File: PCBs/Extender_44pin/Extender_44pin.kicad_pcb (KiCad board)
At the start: 2 copper layers, 119.1 x 224.9 mm, 46 parts, among them J10 J, J11 K, J12 L, J13 M, J14 N, J15 P, J16 R, J17 S, J18 T, J19 U, J20 V, J21 W, J22 X, J23 1, J24 2, J25 3, J26 4, J27 5, J28 6, J29 7, J3 A, J30 8, J31 9, J32 10, J33 11, J34 12, J35 13, J36 14, J37 15, J38 16, J39 17, J4 B, J40 18, J41 19, J42 20, J43 21, J44 22, J45 Y, J46 Z, J5 C, J6 D, J7 E, J8 F, J9 H

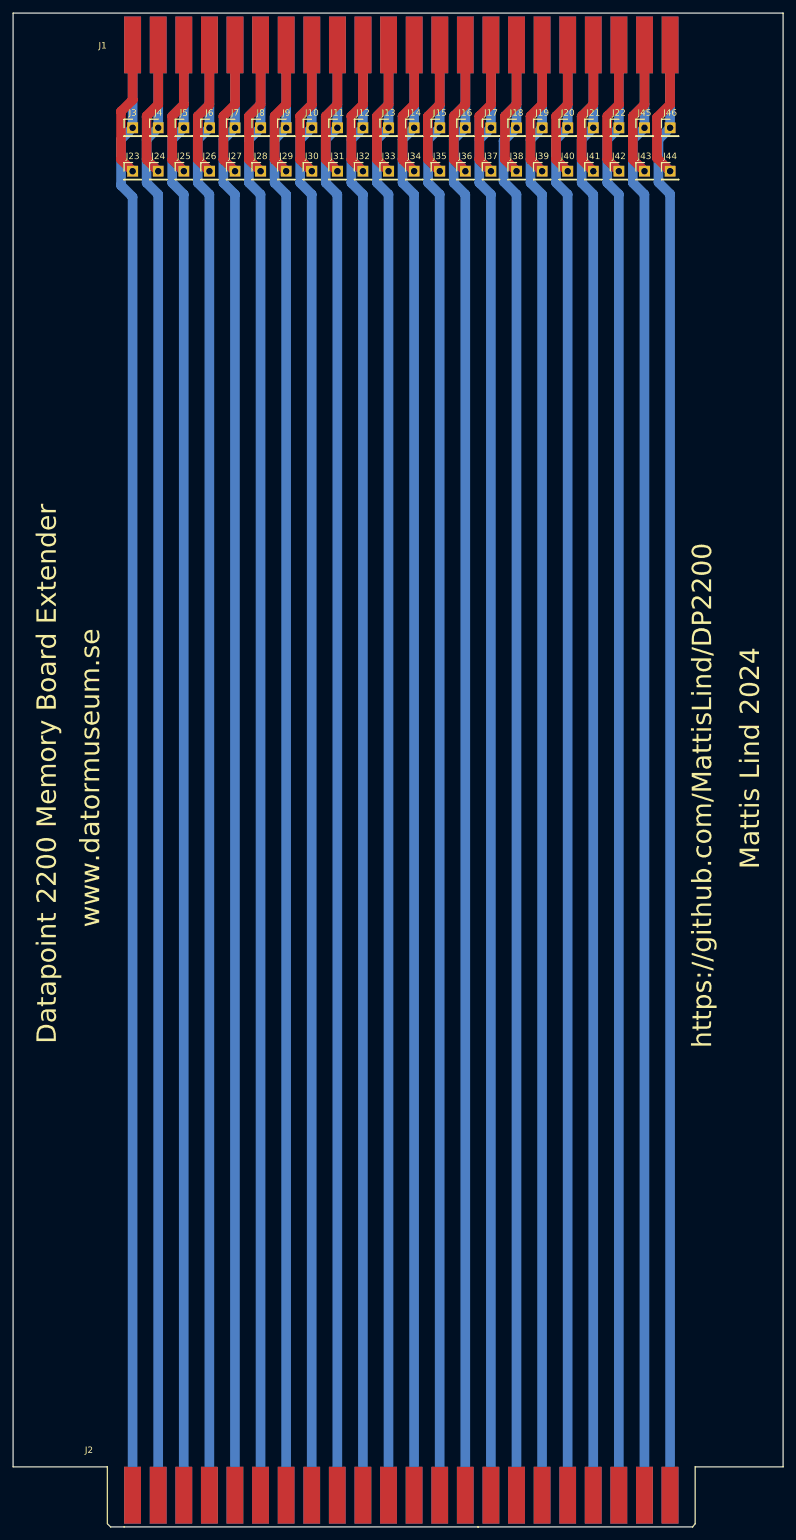
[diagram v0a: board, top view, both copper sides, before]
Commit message: Updates of extender boards.
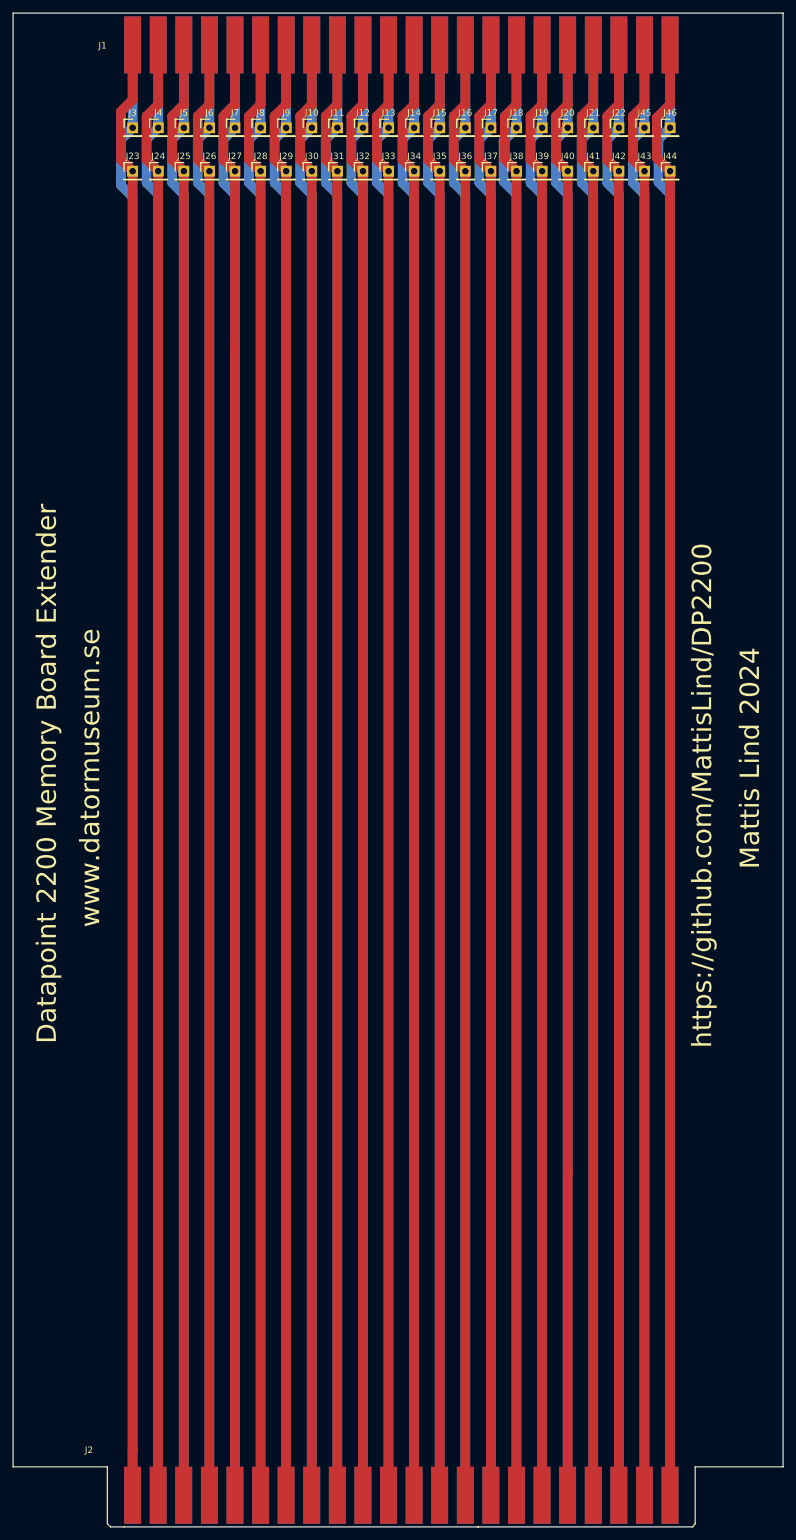
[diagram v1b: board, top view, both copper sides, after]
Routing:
- net /1: track 21.0 -> 225.9 mm
- net /7: track 21.0 -> 225.9 mm
- net /6: track 21.0 -> 225.9 mm
- net /5: track 21.0 -> 225.9 mm
- net /4: track 21.0 -> 225.9 mm
- net /3: track 21.0 -> 225.9 mm
- net /22: track 21.2 -> 226.1 mm
- net /21: track 21.0 -> 225.9 mm
- net /20: track 21.0 -> 225.9 mm
- net /2: track 21.0 -> 225.9 mm
- net /18: track 21.0 -> 225.9 mm
- net /14: track 21.0 -> 225.9 mm
- net /11: track 21.0 -> 225.9 mm
- net /10: track 21.0 -> 225.9 mm
- net /9: track 21.0 -> 225.9 mm
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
